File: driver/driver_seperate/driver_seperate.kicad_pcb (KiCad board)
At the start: 4 copper layers, 37.8 x 34.2 mm, 21 parts, among them IC1 MCT8316Z0TQRGFRQ1, J2 Motor, J3 Conn_01x05, J4 Conn_01x02

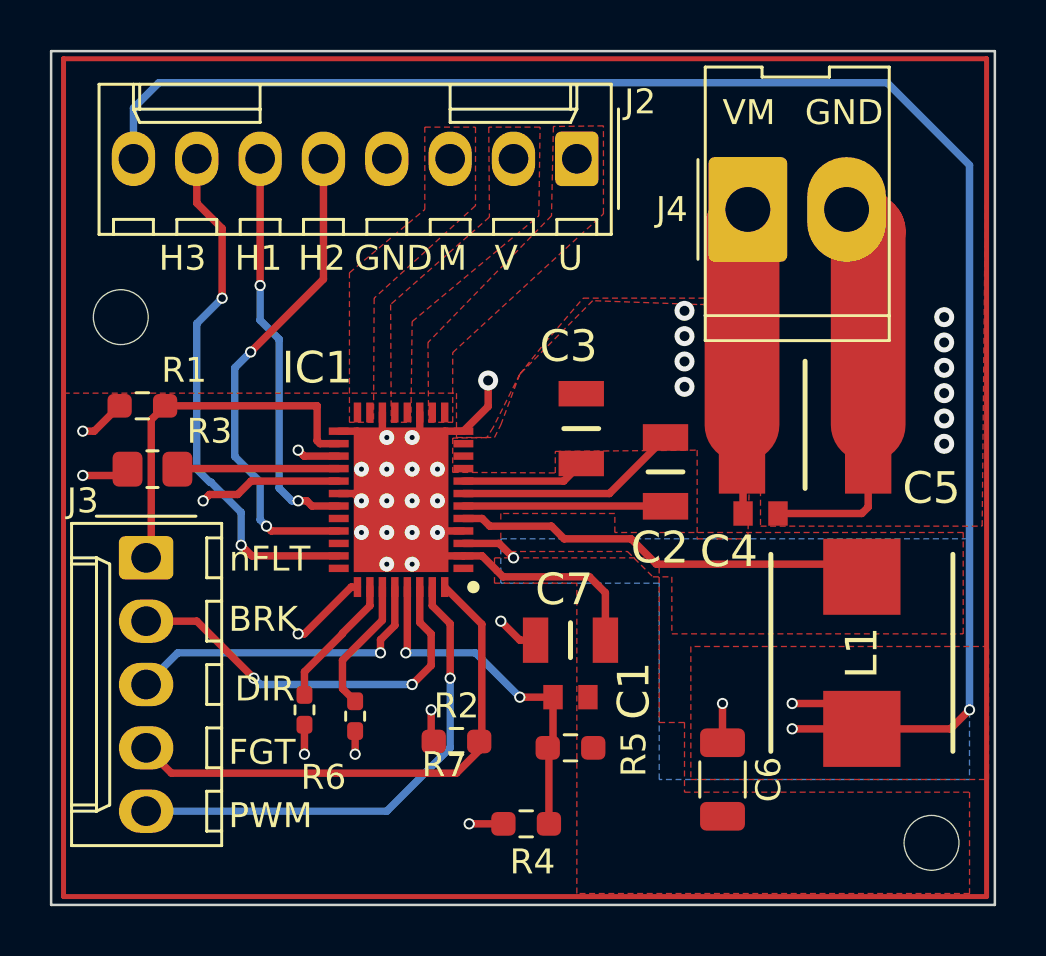
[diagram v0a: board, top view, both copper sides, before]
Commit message: Add pcb v2, Remove old files
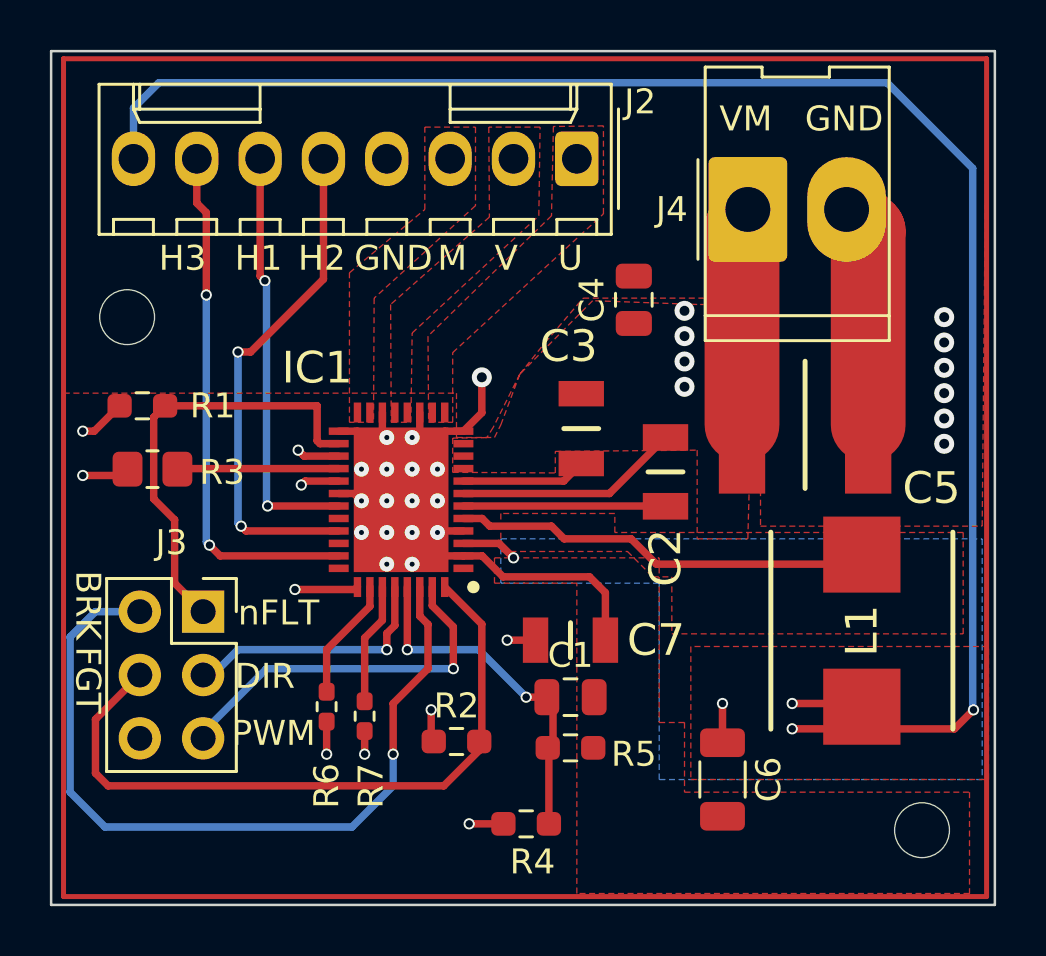
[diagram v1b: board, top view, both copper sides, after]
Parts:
- C1, C4: footprint SamacSys_Parts:CAPC1608X95N -> Capacitor_SMD:C_0805_2012Metric
- C5: value >=10uF -> KCM55TR71H226MH01L
- J3: footprint Connector_Molex:Molex_KK-254_AE-6410-05A_1x05_P2.54mm_Vertical -> Connector_PinSocket_2.54mm:PinSocket_2x03_P2.54mm_Vertical
- moved C4 9.96 mm to (132.3, 74.0), turned to 90 degrees
- moved J3 3.14 mm to (115.1, 86.5), turned to 0 degrees
- moved R6 0.90 mm to (120.0, 90.3)
- moved L1 0.89 mm to (141.5, 87.2)
- moved H1 0.63 mm to (143.9, 95.2)
- moved R7 0.38 mm to (121.5, 90.7)
- moved H2 0.25 mm to (112.0, 74.7)
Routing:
- net /Motor Driver/BRAKE: track 16.1 -> 32.3 mm, vias 2 -> 1
- net GND: track 52.7 -> 45.7 mm
- net /Motor Driver/FGOUT: track 21.4 -> 28.1 mm
- net /Motor Driver/AVDD: track 20.9 -> 15.7 mm
- net /Motor Driver/PWM: track 20.0 -> 15.0 mm
- net /Motor Driver/VM: track 18.8 -> 15.3 mm
- net /Motor Driver/nFault: track 14.8 -> 17.7 mm
- net /Motor Driver/DIR: track 12.8 -> 10.4 mm
- net /Motor Driver/H2: track 19.7 -> 20.5 mm
- net /Motor Driver/H1: track 16.2 -> 16.9 mm
- net /Motor Driver/SW_BK: track 73.7 -> 74.3 mm
- net Net-(IC1-ADVANCE): track 5.45 -> 4.88 mm
